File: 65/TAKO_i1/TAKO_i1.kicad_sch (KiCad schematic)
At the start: 164 parts, among them J1 Conn_01x19_Pin, J2 Conn_01x19_Pin, SW1 MX_SW_solder, SW10 MX_SW_solder, SW11 MX_SW_solder, SW12 MX_SW_solder, SW13 MX_SW_solder, SW14 MX_SW_solder, SW15 MX_SW_solder, SW16 MX_SW_solder, SW17 MX_SW_solder, SW18 MX_SW_solder, SW19 MX_SW_solder, SW2 MX_SW_solder, SW20 MX_SW_solder, SW21 MX_SW_solder, SW22 MX_SW_solder, SW23 MX_SW_solder, SW24 MX_SW_solder, SW25 MX_SW_solder, SW26 MX_SW_solder, SW27 MX_SW_solder, SW28 MX_SW_solder, SW29 MX_SW_solder, SW3 MX_SW_solder, SW30 MX_SW_solder, SW31 MX_SW_solder, SW32 RotaryEncoder_Switch, SW33 MX_SW_solder, SW34 MX_SW_solder, SW35 MX_SW_solder, SW36 MX_SW_solder, SW37 MX_SW_solder, SW38 MX_SW_solder, SW39 MX_SW_solder, SW4 MX_SW_solder, SW40 MX_SW_solder, SW41 MX_SW_solder, SW42 MX_SW_solder, SW43 MX_SW_solder, SW44 MX_SW_solder, SW45 MX_SW_solder, SW46 MX_SW_solder, SW47 MX_SW_solder, SW48 RotaryEncoder_Switch, SW49 MX_SW_solder, SW5 MX_SW_solder, SW50 MX_SW_solder, SW51 MX_SW_solder, SW52 MX_SW_solder, SW53 MX_SW_solder, SW54 MX_SW_solder, SW55 MX_SW_solder, SW56 MX_SW_solder, SW57 MX_SW_solder, SW58 MX_SW_solder, SW59 MX_SW_solder, SW6 MX_SW_solder, SW60 MX_SW_solder, SW61 MX_SW_solder, SW62 MX_SW_solder, SW63 MX_SW_solder, SW64 MX_SW_solder, SW65 MX_SW_solder, SW66 MX_SW_solder, SW67 MX_SW_solder, SW68 MX_SW_solder, SW69 MX_SW_solder, SW7 MX_SW_solder, SW70 MX_SW_solder, SW71 MX_SW_solder, SW72 MX_SW_solder, SW73 MX_SW_solder, SW74 MX_SW_solder, SW75 MX_SW_solder, SW76 SW_Push_45deg, SW8 MX_SW_solder, SW9 MX_SW_solder, U1 Bonsai-C4-extended

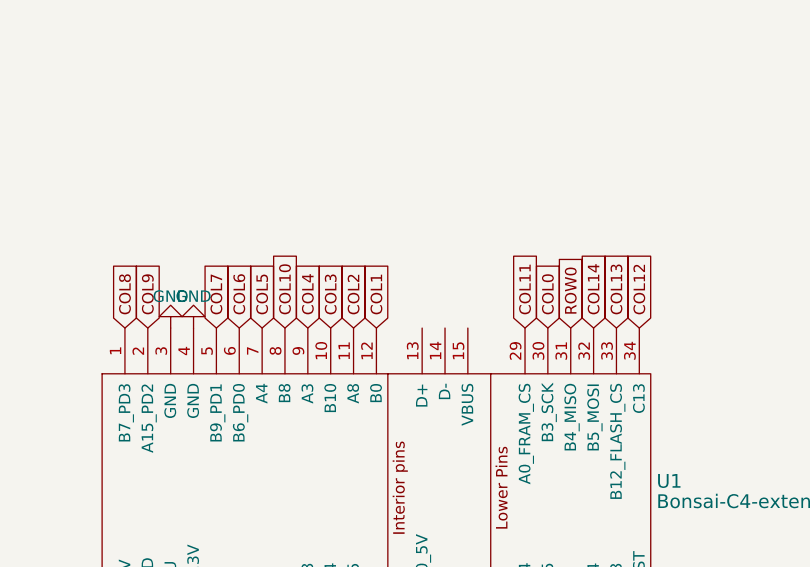
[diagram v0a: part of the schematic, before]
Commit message: working on 60B uni
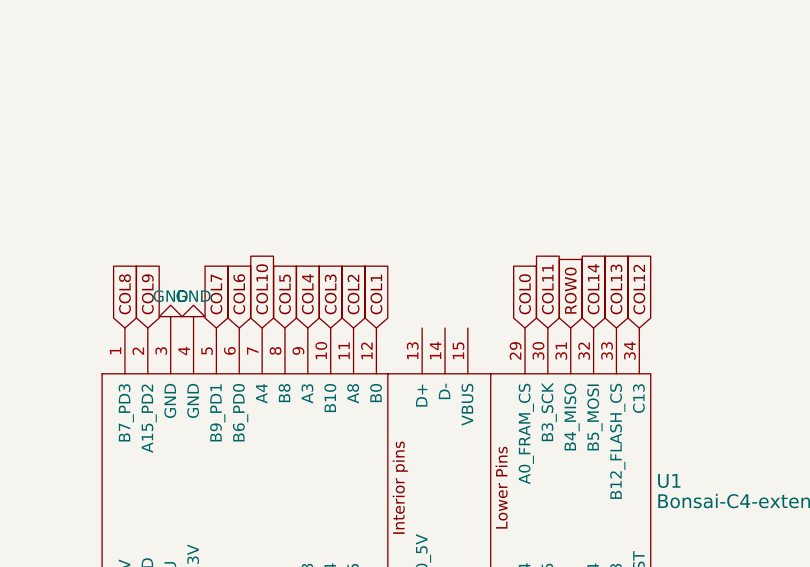
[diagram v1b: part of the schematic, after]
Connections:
- net COL0: now also U1.29 (A0_FRAM_CS); no longer U1.30 (B3_SCK)
- net COL10: now also U1.7 (A4); no longer U1.8 (B8)
- net COL11: now also U1.30 (B3_SCK); no longer U1.29 (A0_FRAM_CS)
- net COL5: now also U1.8 (B8); no longer U1.7 (A4)
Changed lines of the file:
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@@
     )
   )
-  (global_label "COL11" (shape input) (at 95.25 177.8 90) (fields_autoplaced)
+  (global_label "COL11" (shape input) (at 97.79 177.8 90) (fields_autoplaced)
     (effects (font (size 1.27 1.27)) (justify left))
-    (property "Intersheetrefs" "${INTERSHEET_REFS}" (at 95.25 168.8466 90)
-      (effects (font (size 1.27 1.27)) (justify left) hide)
+    (property "Intersheetrefs" "${INTERSHEET_REFS}" (at 97.79 168.8466 90)
+      (effects (font (size 1.27 1.27)) (justify right) hide)
     )
   )
@@
     )
   )
-  (global_label "COL0" (shape input) (at 97.79 177.8 90) (fields_autoplaced)
+  (global_label "COL0" (shape input) (at 95.25 177.8 90) (fields_autoplaced)
     (effects (font (size 1.27 1.27)) (justify left))
-    (property "Intersheetrefs" "${INTERSHEET_REFS}" (at 97.79 170.0561 90)
-      (effects (font (size 1.27 1.27)) (justify left) hide)
+    (property "Intersheetrefs" "${INTERSHEET_REFS}" (at 95.25 170.0561 90)
+      (effects (font (size 1.27 1.27)) (justify right) hide)
     )
   )
@@
     )
   )
-  (global_label "COL10" (shape input) (at 68.58 177.8 90) (fields_autoplaced)
+  (global_label "COL10" (shape input) (at 66.04 177.8 90) (fields_autoplaced)
     (effects (font (size 1.27 1.27)) (justify left))
-    (property "Intersheetrefs" "${INTERSHEET_REFS}" (at 68.58 168.8466 90)
-      (effects (font (size 1.27 1.27)) (justify left) hide)
+    (property "Intersheetrefs" "${INTERSHEET_REFS}" (at 66.04 168.8466 90)
+      (effects (font (size 1.27 1.27)) (justify right) hide)
     )
   )
@@
     )
   )
-  (global_label "COL5" (shape input) (at 66.04 177.8 90) (fields_autoplaced)
+  (global_label "COL5" (shape input) (at 68.58 177.8 90) (fields_autoplaced)
     (effects (font (size 1.27 1.27)) (justify left))
-    (property "Intersheetrefs" "${INTERSHEET_REFS}" (at 66.04 170.0561 90)
-      (effects (font (size 1.27 1.27)) (justify right) hide)
+    (property "Intersheetrefs" "${INTERSHEET_REFS}" (at 68.58 170.0561 90)
+      (effects (font (size 1.27 1.27)) (justify left) hide)
     )
   )
